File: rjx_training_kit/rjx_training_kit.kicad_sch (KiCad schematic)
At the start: 4 parts

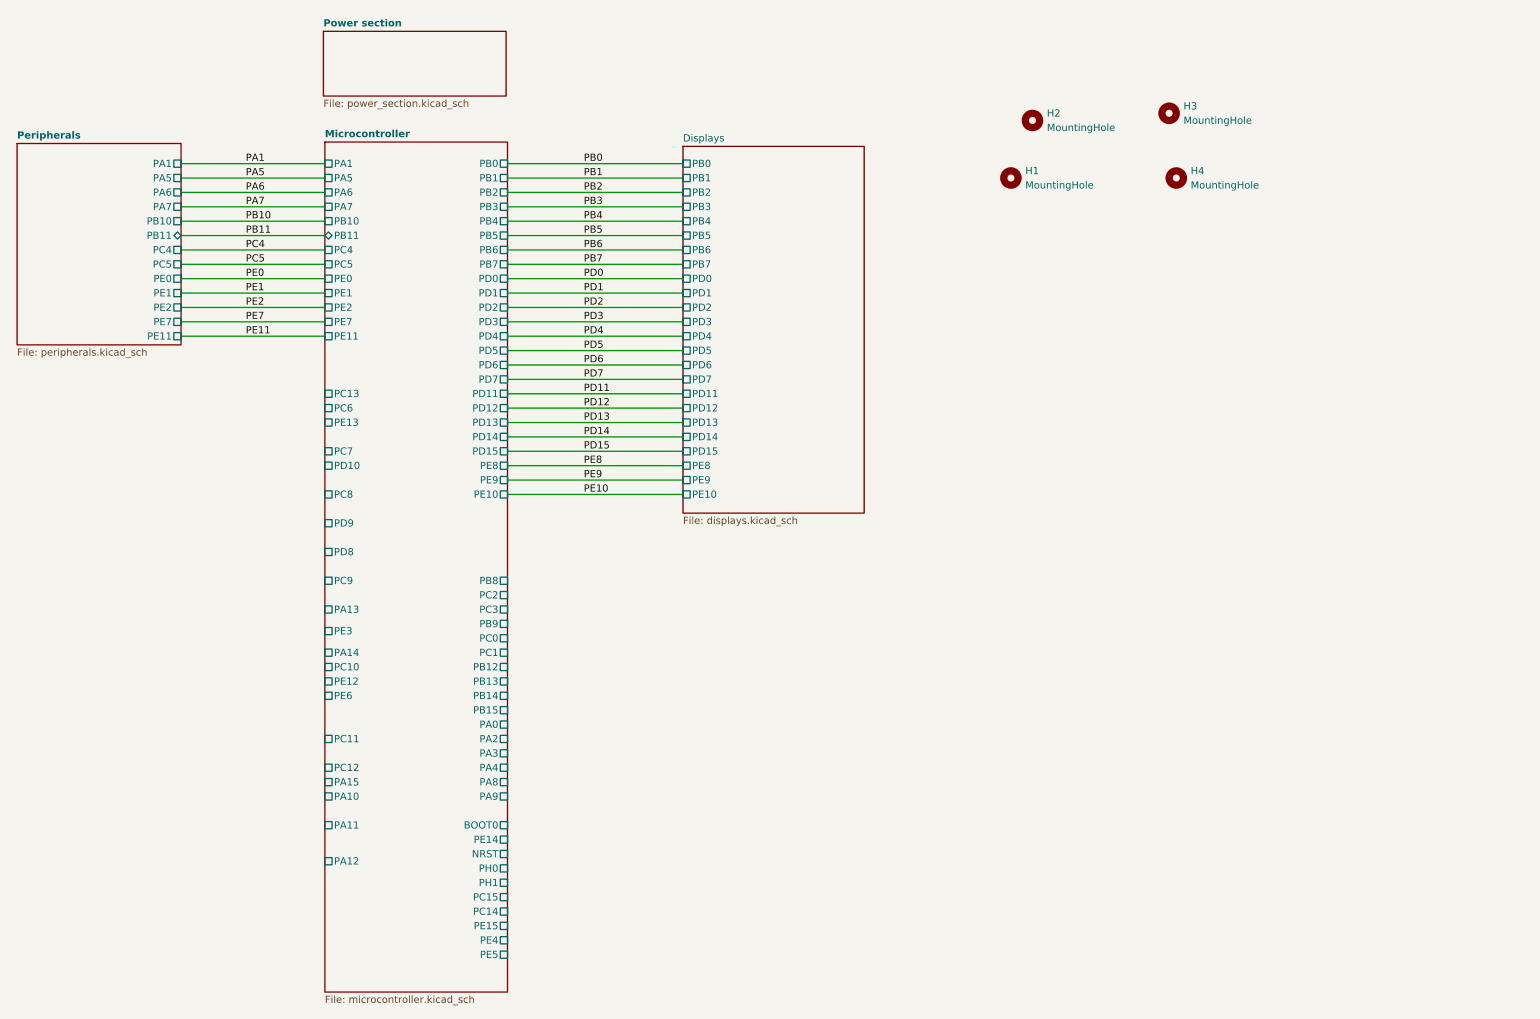
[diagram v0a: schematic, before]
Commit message: Update
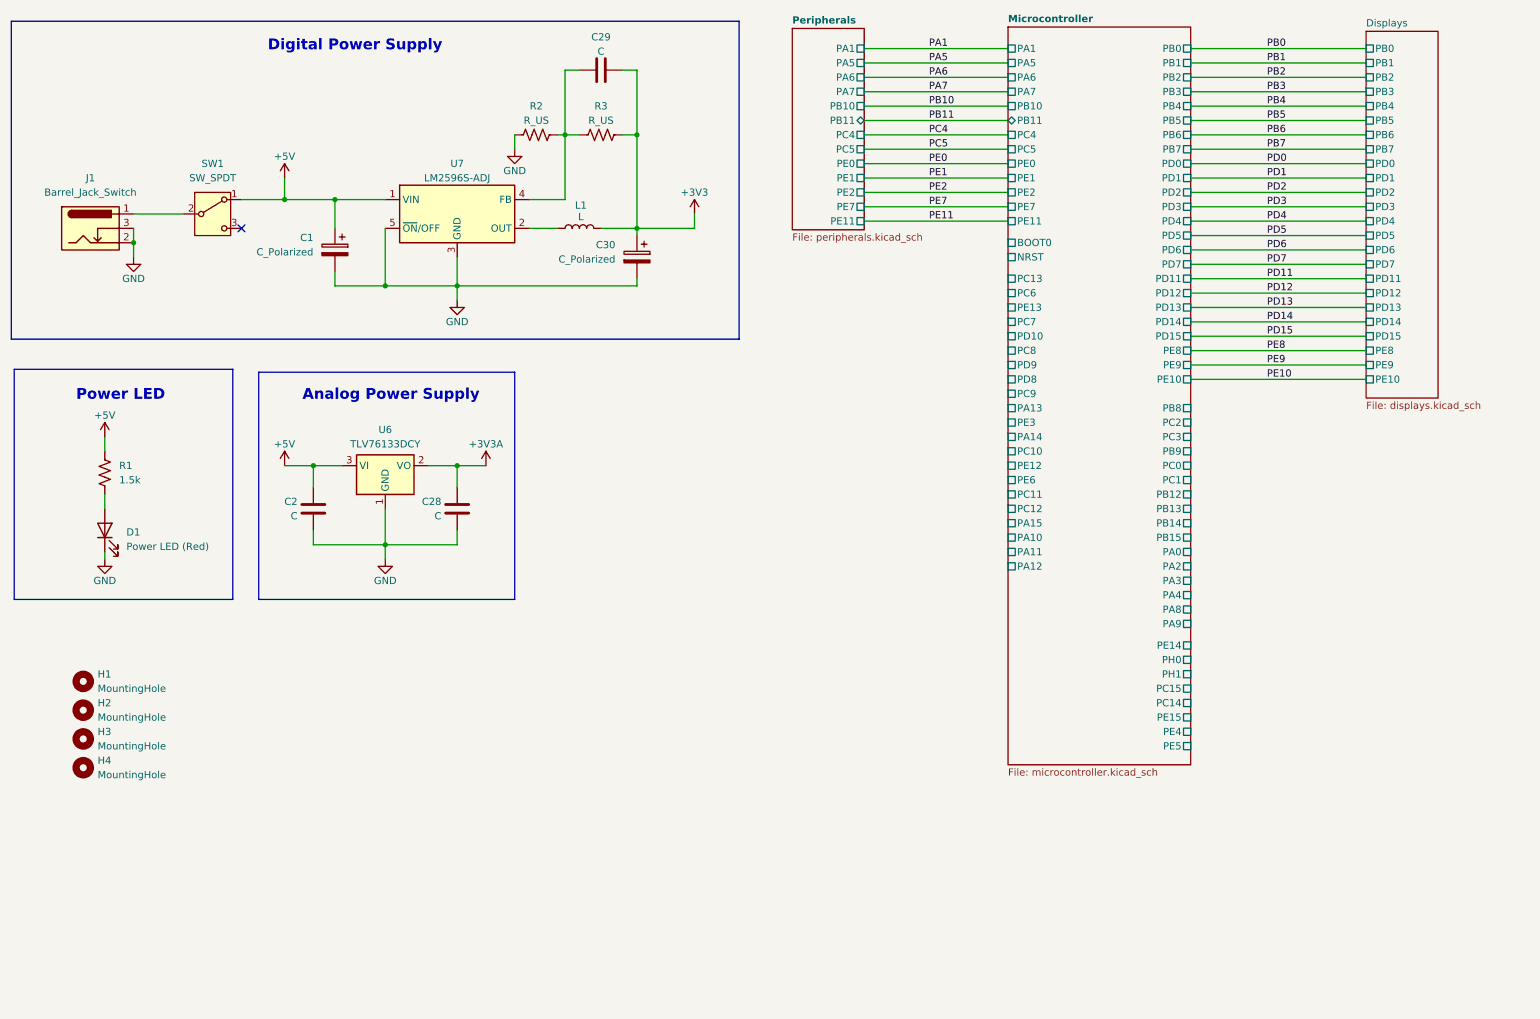
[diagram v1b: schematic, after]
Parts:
- added C1, C30: C_Polarized, symbol Device:C_Polarized
- added C2, C28, C29: C, symbol Device:C
- added D1: Power LED (Red), symbol Device:LED
- added J1: Barrel_Jack_Switch, symbol Connector:Barrel_Jack_Switch
- added L1: L, symbol Device:L
- added R1: 1.5k, symbol Device:R_US
- added R2, R3: R_US, symbol Device:R_US
- added SW1: SW_SPDT, symbol Switch:SW_SPDT
- added U6: TLV76133DCY, Package_TO_SOT_SMD:SOT-223-3_TabPin2, symbol Regulator_Linear:TLV76133DCY
- added U7: LM2596S-ADJ, Package_TO_SOT_SMD:TO-263-5_TabPin3, symbol Regulator_Switching:LM2596S-ADJ
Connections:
- new net: L1.2, U7.2 (OUT)
- new net: C29.1, R2.2, R3.1, U7.4 (FB)
- new net: J1.1, SW1.2 (B)
- new net: D1.2 (A), R1.2
- new net +3V3: C29.2, C30.1, L1.1, R3.2
- new net +3V3A: C28.1, U6.2 (VO)
- new net +5V: C1.1, C2.1, R1.1, SW1.1 (A), U6.3 (VI), U7.1 (VIN)
- new net GND: C1.2, C2.2, C28.2, C30.2, D1.1 (K), J1.2, J1.3, R2.1, U6.1 (GND), U7.3 (GND), U7.5 (~{ON}/OFF)
- no-connect marks 0 -> 1
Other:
- removed sheet Power section
- note added: "Analog Power Supply"
- note added: "Digital Power Supply"
- note added: "Power LED"
- moved on the sheet: H1, H2, H3, H4
